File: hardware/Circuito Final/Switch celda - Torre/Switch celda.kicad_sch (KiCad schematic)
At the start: 28 parts, among them Q1 MMBT2222A, Q2 MMBT2907A, Q3 MMBT2222A

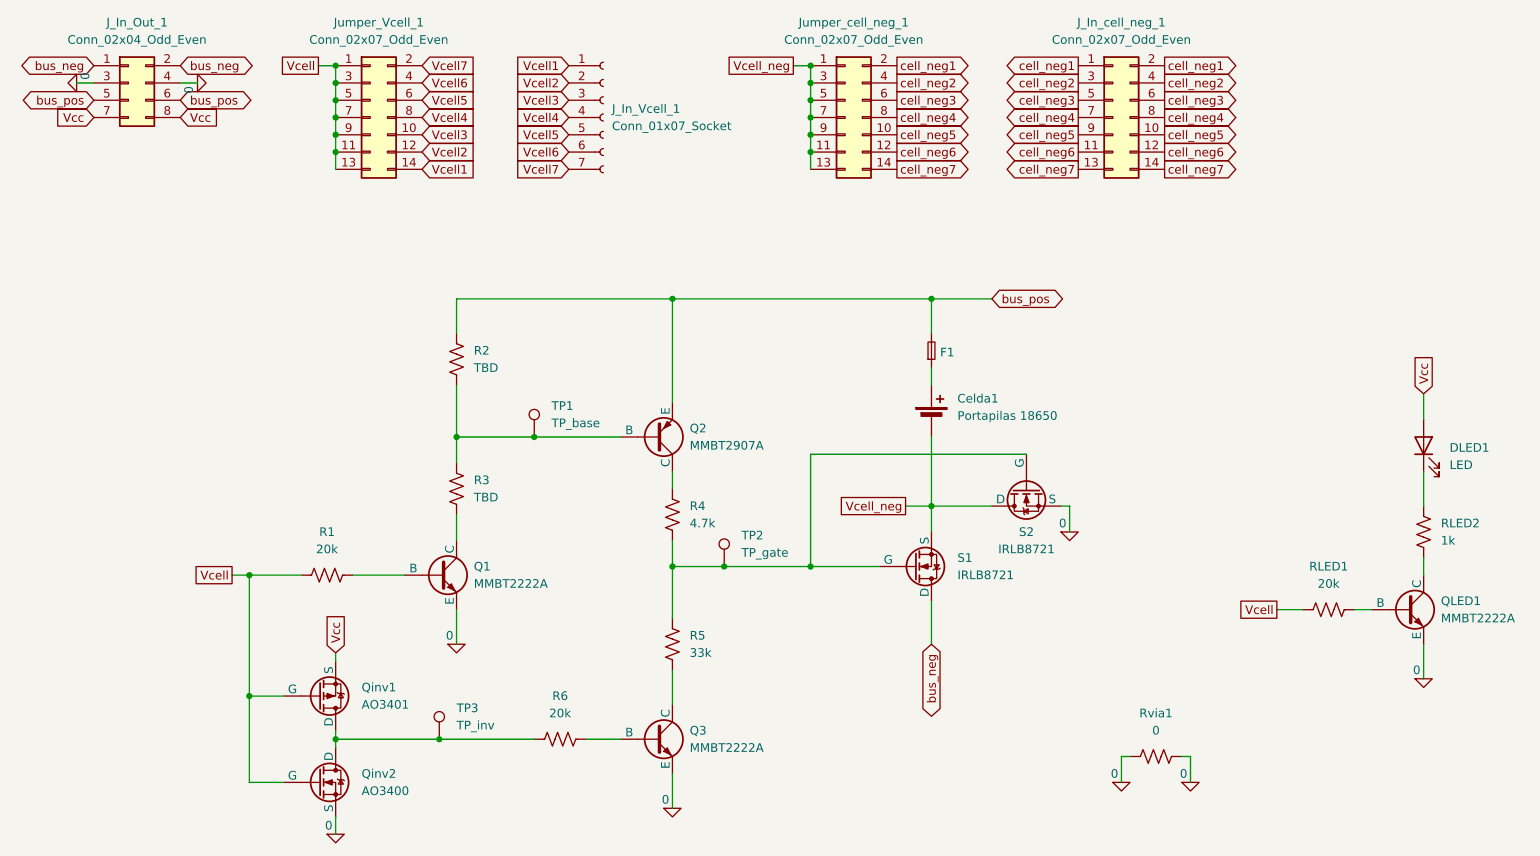
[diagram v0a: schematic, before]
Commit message: update pcb celdas
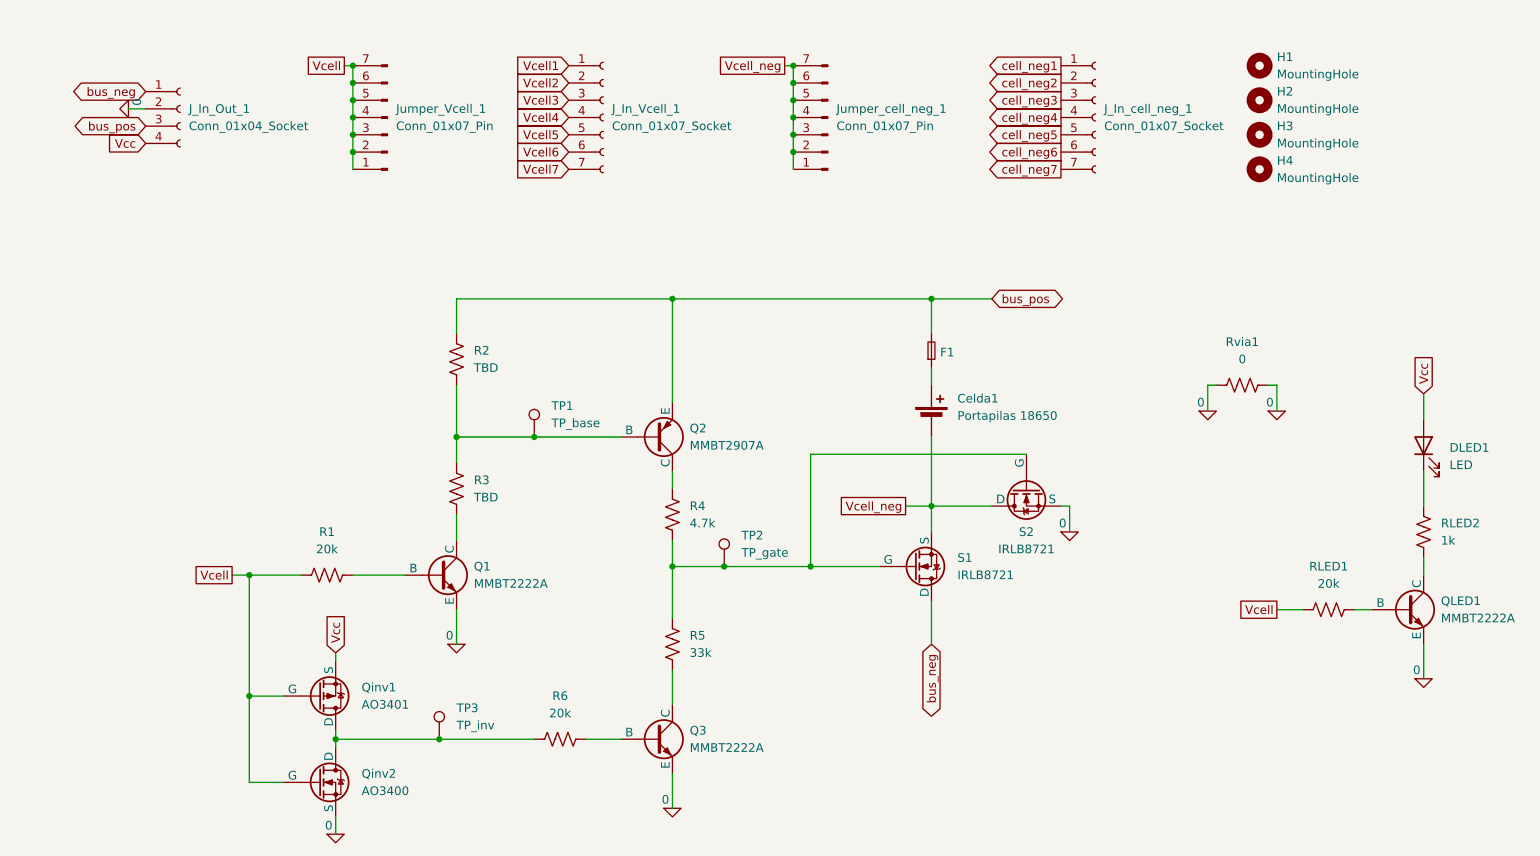
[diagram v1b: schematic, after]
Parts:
- removed J_In_Out_1: Conn_02x04_Odd_Even, Connector_PinSocket_2.54mm:PinSocket_2x04_P2.54mm_Vertical, symbol Connector_Generic:Conn_02x04_Odd_Even
- removed J_In_cell_neg_1, Jumper_Vcell_1, Jumper_cell_neg_1: Conn_02x07_Odd_Even, Connector_PinSocket_2.54mm:PinSocket_2x07_P2.54mm_Vertical, symbol Connector_Generic:Conn_02x07_Odd_Even
- added H1, H2, H3, H4: MountingHole, MountingHole:MountingHole_3.5mm, symbol Mechanical:MountingHole
- added J_In_Out_1: Conn_01x04_Socket, symbol Connector:Conn_01x04_Socket
- added J_In_cell_neg_1: Conn_01x07_Socket, Connector_PinSocket_2.54mm:PinSocket_1x07_P2.54mm_Vertical, symbol Connector:Conn_01x07_Socket
- added Jumper_Vcell_1, Jumper_cell_neg_1: Conn_01x07_Pin, Connector_PinHeader_2.54mm:PinHeader_1x07_P2.54mm_Vertical, symbol Connector:Conn_01x07_Pin
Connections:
- net 0: now also J_In_Out_1.2 (Pin_2)
- net Vcc: now also J_In_Out_1.4 (Pin_4)
- net Vcell: now also Jumper_Vcell_1.1 (Pin_1), Jumper_Vcell_1.2 (Pin_2), Jumper_Vcell_1.3 (Pin_3), Jumper_Vcell_1.4 (Pin_4), Jumper_Vcell_1.5 (Pin_5), Jumper_Vcell_1.6 (Pin_6), Jumper_Vcell_1.7 (Pin_7)
- net Vcell_neg: now also Jumper_cell_neg_1.1 (Pin_1), Jumper_cell_neg_1.2 (Pin_2), Jumper_cell_neg_1.3 (Pin_3), Jumper_cell_neg_1.4 (Pin_4), Jumper_cell_neg_1.5 (Pin_5), Jumper_cell_neg_1.6 (Pin_6), Jumper_cell_neg_1.7 (Pin_7)
- net bus_neg: now also J_In_Out_1.1 (Pin_1)
- net bus_pos: now also J_In_Out_1.3 (Pin_3)
- net cell_neg1: now also J_In_cell_neg_1.1 (Pin_1)
- net cell_neg2: now also J_In_cell_neg_1.2 (Pin_2)
- net cell_neg3: now also J_In_cell_neg_1.3 (Pin_3)
- net cell_neg4: now also J_In_cell_neg_1.4 (Pin_4)
- net cell_neg5: now also J_In_cell_neg_1.5 (Pin_5)
- net cell_neg6: now also J_In_cell_neg_1.6 (Pin_6)
- net cell_neg7: now also J_In_cell_neg_1.7 (Pin_7)
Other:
- moved on the sheet: Rvia1
